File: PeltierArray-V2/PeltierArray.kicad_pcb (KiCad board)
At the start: 2 copper layers, 100 x 100 mm, 13 parts, among them J1 Barrel_Jack

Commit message: TB6612
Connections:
- net /STBY renamed STBY

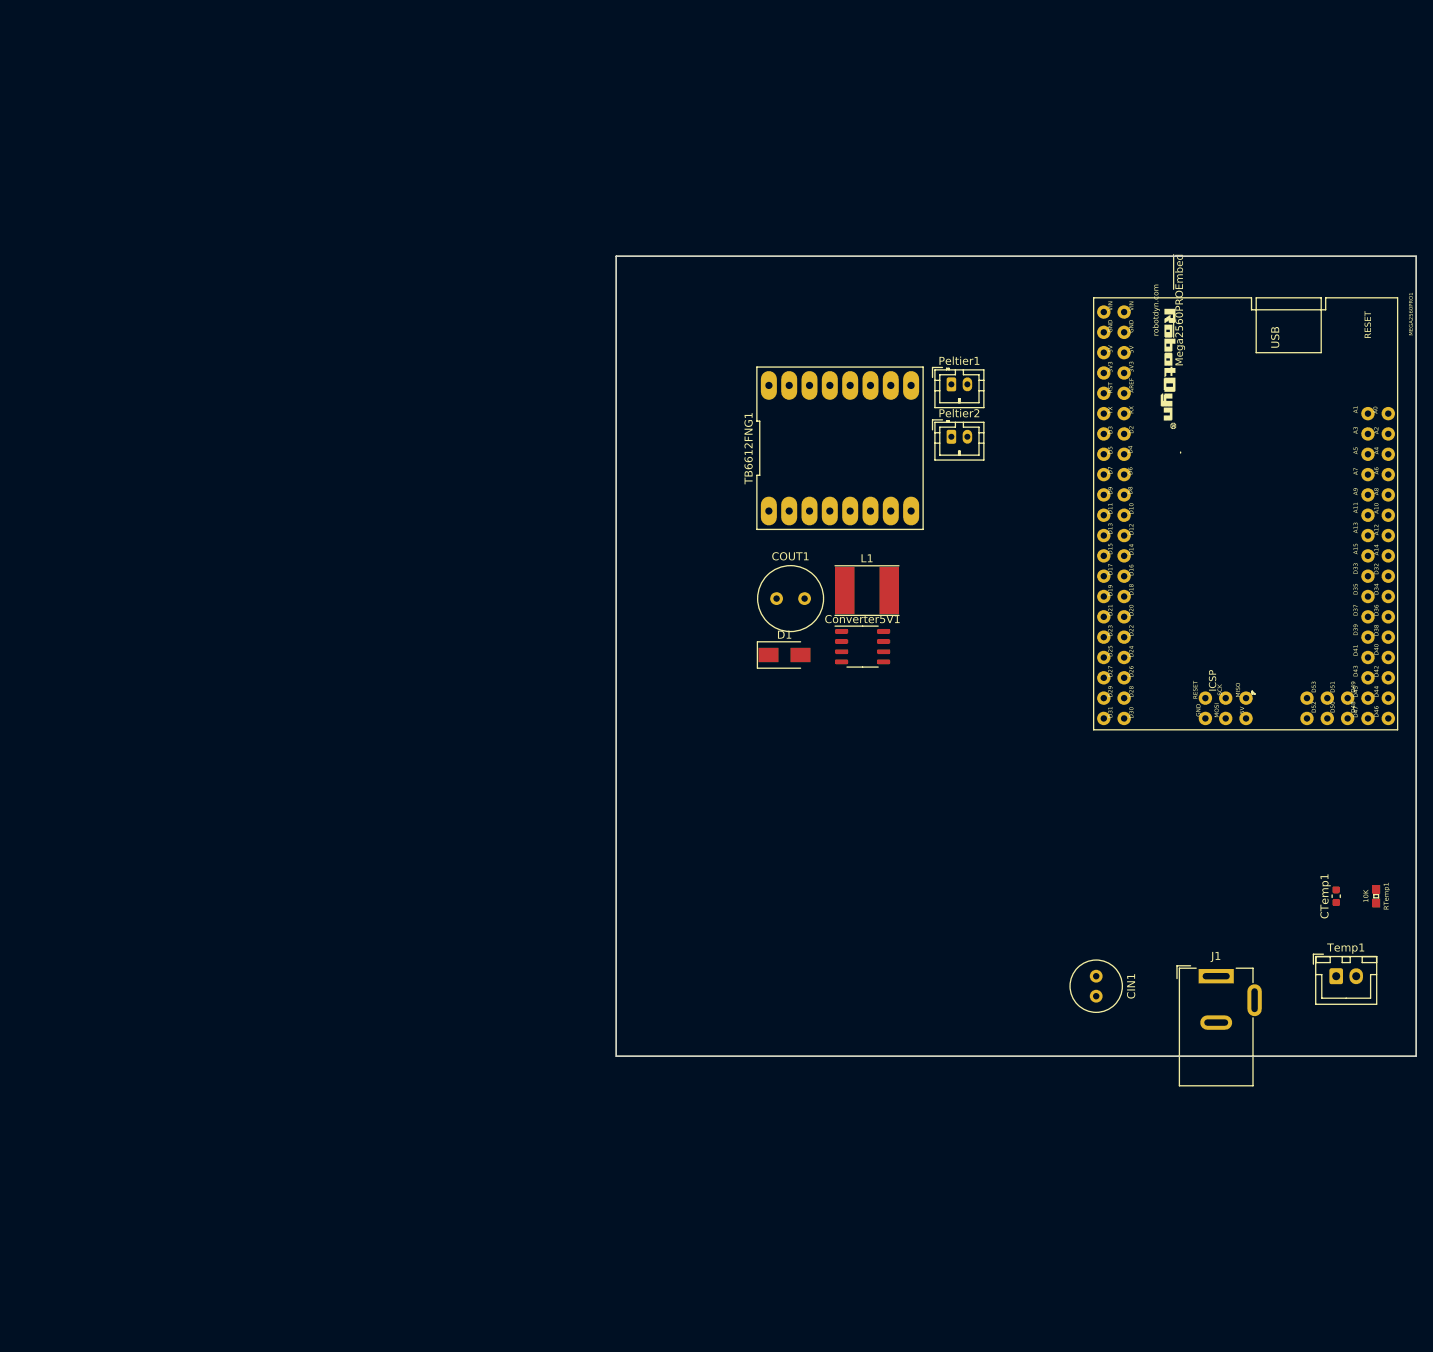
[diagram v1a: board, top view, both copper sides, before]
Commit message: UART I2C
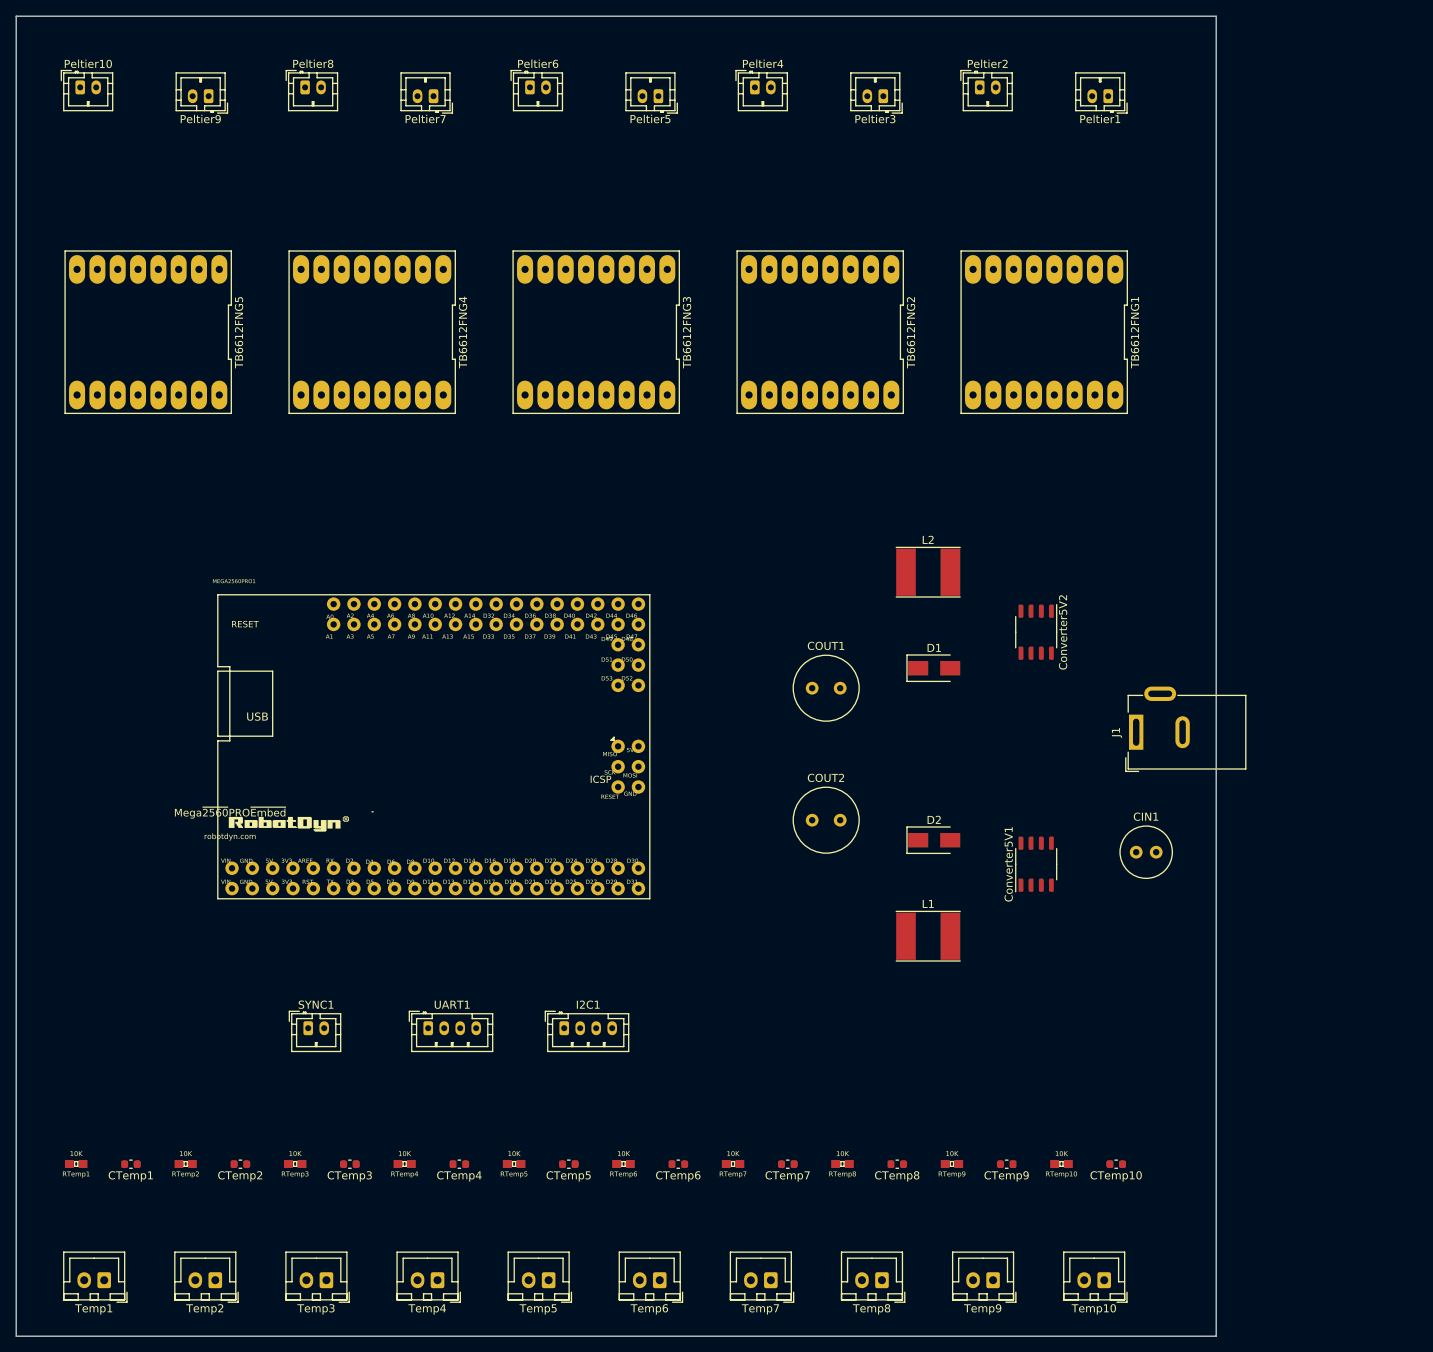
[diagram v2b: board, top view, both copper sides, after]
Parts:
- added COUT2: CP330uF25V, Capacitor_THT:C_Radial_D8.0mm_H11.5mm_P3.50mm, F.Cu at (124.5, 120.5)
- added CTemp10: 100nF, Capacitor_SMD:C_0603_1608Metric, F.Cu at (162.5, 163.5)
- added CTemp2: 100nF, Capacitor_SMD:C_0603_1608Metric, F.Cu at (53.0, 163.5)
- added CTemp3: 100nF, Capacitor_SMD:C_0603_1608Metric, F.Cu at (66.7, 163.5)
- added CTemp4: 100nF, Capacitor_SMD:C_0603_1608Metric, F.Cu at (80.4, 163.5)
- added CTemp5: 100nF, Capacitor_SMD:C_0603_1608Metric, F.Cu at (94.1, 163.5)
- added CTemp6: 100nF, Capacitor_SMD:C_0603_1608Metric, F.Cu at (107.8, 163.5)
- added CTemp7: 100nF, Capacitor_SMD:C_0603_1608Metric, F.Cu at (121.4, 163.5)
- added CTemp8: 100nF, Capacitor_SMD:C_0603_1608Metric, F.Cu at (135.1, 163.5)
- added CTemp9: 100nF, Capacitor_SMD:C_0603_1608Metric, F.Cu at (148.8, 163.5)
- added Converter5V2: TD1509, Package_SO:SOP-8_3.9x4.9mm_P1.27mm, F.Cu at (152.5, 97.0)
- added D2: D_Schottky, Diode_SMD:D_SMA, F.Cu at (139.8, 123.0)
- added I2C1: Conn_01x04_Male, Connector_JST:JST_PH_B4B-PH-K_1x04_P2.00mm_Vertical, F.Cu at (93.5, 146.5)
- added L2: L 33uF 4.5A, Inductor_SMD:L_Taiyo-Yuden_NR-60xx_HandSoldering, F.Cu at (139.0, 89.5)
- added Peltier10: Conn_01x02_Male, Connector_JST:JST_PH_B2B-PH-K_1x02_P2.00mm_Vertical, F.Cu at (33.0, 28.9)
- added Peltier3: Conn_01x02_Male, Connector_JST:JST_PH_B2B-PH-K_1x02_P2.00mm_Vertical, F.Cu at (133.4, 30.0)
- added Peltier4: Conn_01x02_Male, Connector_JST:JST_PH_B2B-PH-K_1x02_P2.00mm_Vertical, F.Cu at (117.3, 28.9)
- added Peltier5: Conn_01x02_Male, Connector_JST:JST_PH_B2B-PH-K_1x02_P2.00mm_Vertical, F.Cu at (105.3, 30.0)
- added Peltier6: Conn_01x02_Male, Connector_JST:JST_PH_B2B-PH-K_1x02_P2.00mm_Vertical, F.Cu at (89.2, 28.9)
- added Peltier7: Conn_01x02_Male, Connector_JST:JST_PH_B2B-PH-K_1x02_P2.00mm_Vertical, F.Cu at (77.2, 30.0)
- added Peltier8: Conn_01x02_Male, Connector_JST:JST_PH_B2B-PH-K_1x02_P2.00mm_Vertical, F.Cu at (61.1, 28.9)
- added Peltier9: Conn_01x02_Male, Connector_JST:JST_PH_B2B-PH-K_1x02_P2.00mm_Vertical, F.Cu at (49.1, 30.0)
- added RTemp10: 10K, Resistors:0603, F.Cu at (155.7, 163.5)
- added RTemp2: 10K, Resistors:0603, F.Cu at (46.2, 163.5)
- added RTemp3: 10K, Resistors:0603, F.Cu at (59.9, 163.5)
- added RTemp4: 10K, Resistors:0603, F.Cu at (73.6, 163.5)
- added RTemp5: 10K, Resistors:0603, F.Cu at (87.2, 163.5)
- added RTemp6: 10K, Resistors:0603, F.Cu at (100.9, 163.5)
- added RTemp7: 10K, Resistors:0603, F.Cu at (114.6, 163.5)
- added RTemp8: 10K, Resistors:0603, F.Cu at (128.3, 163.5)
- added RTemp9: 10K, Resistors:0603, F.Cu at (142.0, 163.5)
- added SYNC1: Conn_01x02_Male, Connector_JST:JST_PH_B2B-PH-K_1x02_P2.00mm_Vertical, F.Cu at (61.5, 146.5)
- added TB6612FNG2: TB6612FNG, PeltierArray:DIP-16_617_ELL, F.Cu at (125.5, 59.5)
- added TB6612FNG3: TB6612FNG, PeltierArray:DIP-16_617_ELL, F.Cu at (97.5, 59.5)
- added TB6612FNG4: TB6612FNG, PeltierArray:DIP-16_617_ELL, F.Cu at (69.5, 59.5)
- added TB6612FNG5: TB6612FNG, PeltierArray:DIP-16_617_ELL, F.Cu at (41.5, 59.5)
- added Temp10: Conn_01x02_Male, Connector_JST:JST_XH_B2B-XH-A_1x02_P2.50mm_Vertical, F.Cu at (161.0, 178.0)
- added Temp2: Conn_01x02_Male, Connector_JST:JST_XH_B2B-XH-A_1x02_P2.50mm_Vertical, F.Cu at (49.9, 178.0)
- added Temp3: Conn_01x02_Male, Connector_JST:JST_XH_B2B-XH-A_1x02_P2.50mm_Vertical, F.Cu at (63.8, 178.0)
- added Temp4: Conn_01x02_Male, Connector_JST:JST_XH_B2B-XH-A_1x02_P2.50mm_Vertical, F.Cu at (77.7, 178.0)
- added Temp5: Conn_01x02_Male, Connector_JST:JST_XH_B2B-XH-A_1x02_P2.50mm_Vertical, F.Cu at (91.6, 178.0)
- added Temp6: Conn_01x02_Male, Connector_JST:JST_XH_B2B-XH-A_1x02_P2.50mm_Vertical, F.Cu at (105.4, 178.0)
- added Temp7: Conn_01x02_Male, Connector_JST:JST_XH_B2B-XH-A_1x02_P2.50mm_Vertical, F.Cu at (119.3, 178.0)
- added Temp8: Conn_01x02_Male, Connector_JST:JST_XH_B2B-XH-A_1x02_P2.50mm_Vertical, F.Cu at (133.2, 178.0)
- added Temp9: Conn_01x02_Male, Connector_JST:JST_XH_B2B-XH-A_1x02_P2.50mm_Vertical, F.Cu at (147.1, 178.0)
- added UART1: Conn_01x04_Male, Connector_JST:JST_PH_B4B-PH-K_1x04_P2.00mm_Vertical, F.Cu at (76.5, 146.5)
- moved RTemp1 165.9 mm to (32.5, 163.5), turned to 180 degrees
- moved Temp1 158.6 mm to (36.0, 178.0), turned to 180 degrees
- moved CTemp1 154.3 mm to (39.3, 163.5), turned to 180 degrees
- moved MEGA2560PRO1 97.1 mm to (85.0, 110.0), turned to 0 degrees
- moved L1 43.9 mm to (139.0, 135.0)
- moved Peltier2 43.8 mm to (145.4, 28.9)
- moved Peltier1 41.0 mm to (161.5, 30.0), turned to 180 degrees
- moved Converter5V1 34.8 mm to (152.5, 126.0), turned to 90 degrees
- moved J1 32.1 mm to (165.0, 109.5), turned to 90 degrees
- moved TB6612FNG1 29.4 mm to (153.5, 59.5), turned to 180 degrees
- moved D1 18.8 mm to (139.8, 101.5)
- moved CIN1 16.3 mm to (165.0, 124.5), turned to 0 degrees
- moved COUT1 12.1 mm to (124.5, 104.0)
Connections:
- MEGA2560PRO1 pad A0: (no net) -> /Temp0
- MEGA2560PRO1 pad A2: (no net) -> /Temp2
- MEGA2560PRO1 pad A3: (no net) -> /Temp3
- MEGA2560PRO1 pad A4: (no net) -> /Temp4
- MEGA2560PRO1 pad A5: (no net) -> /Temp5
- MEGA2560PRO1 pad A6: (no net) -> /Temp6
- MEGA2560PRO1 pad A7: (no net) -> /Temp7
- MEGA2560PRO1 pad A8: (no net) -> /Temp8
- MEGA2560PRO1 pad A9: (no net) -> /Temp9
- MEGA2560PRO1 pad D18: (no net) -> /TX1
- MEGA2560PRO1 pad D19: (no net) -> /RX1
- MEGA2560PRO1 pad D20: (no net) -> /SDA
- MEGA2560PRO1 pad D21: (no net) -> /SCL
- MEGA2560PRO1 pad D22: (no net) -> /PWM2
- MEGA2560PRO1 pad D23: (no net) -> /PWM1
- MEGA2560PRO1 pad D24: (no net) -> /A2
- MEGA2560PRO1 pad D25: (no net) -> /A1
- MEGA2560PRO1 pad D26: (no net) -> /B2
- MEGA2560PRO1 pad D27: (no net) -> /B1
- MEGA2560PRO1 pad D28: (no net) -> /PWM4
- MEGA2560PRO1 pad D29: (no net) -> /PWM3
- MEGA2560PRO1 pad D30: (no net) -> /A4
- MEGA2560PRO1 pad D31: (no net) -> /A3
- MEGA2560PRO1 pad D32: (no net) -> /B4
- MEGA2560PRO1 pad D33: (no net) -> /B3
- MEGA2560PRO1 pad D34: (no net) -> /PWM6
- MEGA2560PRO1 pad D35: (no net) -> /PWM5
- MEGA2560PRO1 pad D36: (no net) -> /A6
- MEGA2560PRO1 pad D37: (no net) -> /A5
- MEGA2560PRO1 pad D38: (no net) -> /B6
- MEGA2560PRO1 pad D39: (no net) -> /B5
- MEGA2560PRO1 pad D4: /PWM2 -> /SYNC
- MEGA2560PRO1 pad D40: (no net) -> /PWM8
- MEGA2560PRO1 pad D41: (no net) -> /PWM7
- MEGA2560PRO1 pad D42: (no net) -> /A8
- MEGA2560PRO1 pad D43: (no net) -> /A7
- MEGA2560PRO1 pad D44: (no net) -> /B8
- MEGA2560PRO1 pad D45: (no net) -> /B7
- MEGA2560PRO1 pad D46: (no net) -> /PWM10
- MEGA2560PRO1 pad D47: (no net) -> /PWM9
- MEGA2560PRO1 pad D48: (no net) -> /A10
- MEGA2560PRO1 pad D49: (no net) -> /A9
- MEGA2560PRO1 pad D5: /PWM1 -> (no net)
- MEGA2560PRO1 pad D50: (no net) -> /B10
- MEGA2560PRO1 pad D51: (no net) -> /B9
- MEGA2560PRO1 pad D6: /A2 -> (no net)
- MEGA2560PRO1 pad D7: /A1 -> (no net)
- MEGA2560PRO1 pad D8: /B2 -> (no net)
- MEGA2560PRO1 pad D9: /B1 -> (no net)
- RTemp1 pad 2: /Temp1 -> /Temp8
- TB6612FNG1 pad 10: /B1 -> /B9
- TB6612FNG1 pad 11: /A1 -> /A9
- TB6612FNG1 pad 13: /A2 -> /A10
- TB6612FNG1 pad 14: /B2 -> /B10
- TB6612FNG1 pad 15: /PWM2 -> /PWM10
- TB6612FNG1 pad 9: /PWM1 -> /PWM9
- Temp1 pad 2: /Temp1 -> /Temp8
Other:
- board size 100 x 100 mm -> 150 x 165 mm
